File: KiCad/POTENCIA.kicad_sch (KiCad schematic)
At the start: 23 parts, among them J201 Screw_Terminal_01x04, M4 Motor_DC, M5 Motor_DC, M6 Motor_DC, Q201 IRLZ44N, U5 TB6612FNG, U7 ATtiny1616-M, U8 DRV8871DDA

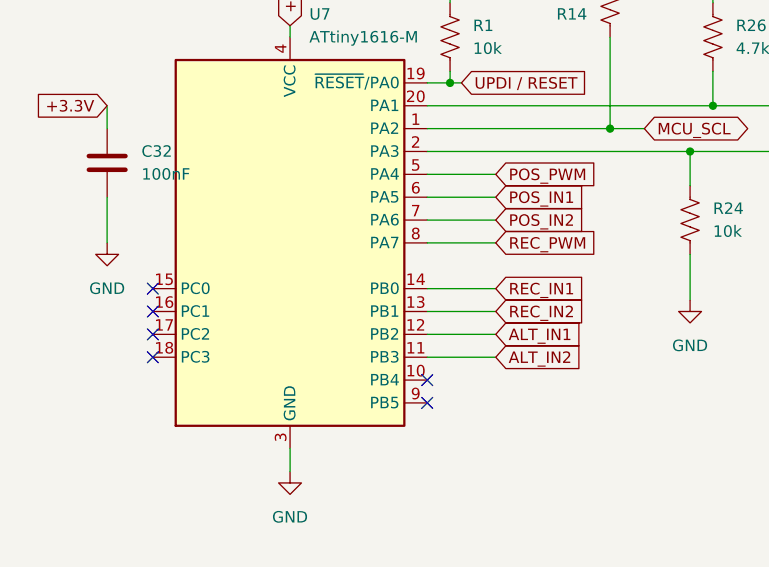
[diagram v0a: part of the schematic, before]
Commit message: Rounting
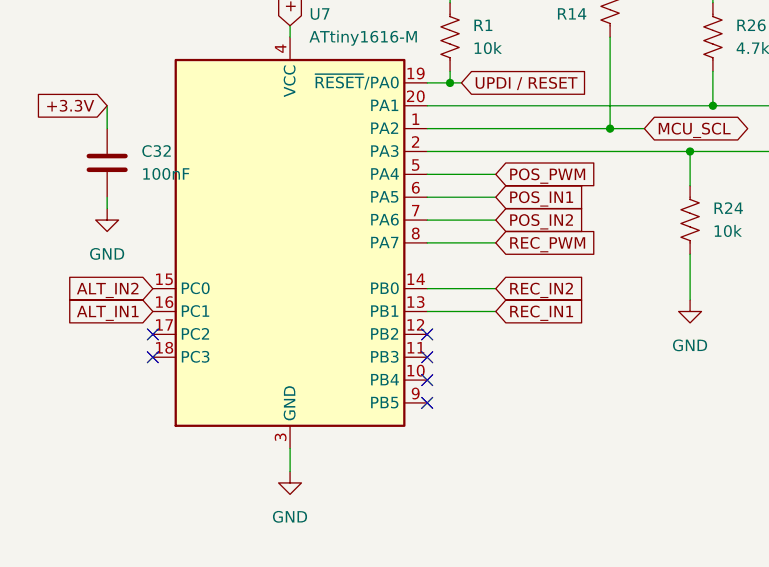
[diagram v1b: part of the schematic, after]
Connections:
- net ALT_IN1: now also U7.16 (PC1); no longer U7.12 (PB2)
- net ALT_IN2: now also U7.15 (PC0); no longer U7.11 (PB3)
- net REC_IN1: now also U7.13 (PB1); no longer U7.14 (PB0)
- net REC_IN2: now also U7.14 (PB0); no longer U7.13 (PB1)
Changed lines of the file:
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@@
 	)
 	(no_connect
-		(at 31.75 152.4)
+		(at 62.23 154.94)
 	)
 	(no_connect
@@
 	)
 	(no_connect
-		(at 31.75 149.86)
-	)
-	(wire
-		(pts
-			(xy 26.67 139.7) (xy 26.67 144.78)
+		(at 62.23 157.48)
+	)
+	(wire
+		(pts
+			(xy 26.67 139.7) (xy 26.67 140.97)
 		)
 		(stroke
@@
 	(wire
 		(pts
-			(xy 62.23 157.48) (xy 69.85 157.48)
-		)
-		(stroke
-			(width 0)
-			(type default)
-		)
-	)
-	(wire
-		(pts
 			(xy 93.98 125.73) (xy 93.98 129.54)
 		)
@@
 		(pts
 			(xy 54.61 88.9) (xy 54.61 95.25)
-		)
-		(stroke
-			(width 0)
-			(type default)
-		)
-	)
-	(wire
-		(pts
-			(xy 62.23 154.94) (xy 69.85 154.94)
 		)
 		(stroke
@@
 	(global_label "REC_IN1"
 		(shape input)
-		(at 69.85 149.86 0)
+		(at 69.85 152.4 0)
 		(fields_autoplaced yes)
 		(effects
@@
 		)
 		(property "Intersheetrefs" "${INTERSHEET_REFS}"
-			(at 80.6366 149.86 0)
+			(at 80.6366 152.4 0)
 			(effects
 				(font
@@
 	(global_label "ALT_IN2"
 		(shape input)
-		(at 69.85 157.48 0)
+		(at 31.75 149.86 180)
+		(fields_autoplaced yes)
+		(effects
+			(font
+				(size 1.27 1.27)
+			)
+			(justify right)
+		)
+		(property "Intersheetrefs" "${INTERSHEET_REFS}"
+			(at 22.2223 149.86 0)
+			(effects
+				(font
+					(size 1.27 1.27)
+				)
+				(justify right)
+				(hide yes)
+			)
+		)
+	)
+	(global_label "VBAT"
+		(shape input)
+		(at 34.29 20.32 180)
+		(fields_autoplaced yes)
+		(effects
+			(font
+				(size 1.27 1.27)
+			)
+			(justify right)
+		)
+		(property "Intersheetrefs" "${INTERSHEET_REFS}"
+			(at 27.5442 20.32 0)
+			(effects
+				(font
+					(size 1.27 1.27)
+				)
+				(justify right)
+				(hide yes)
+			)
+		)
+	)
+	(global_label "POS_IN2"
+		(shape input)
+		(at 69.85 142.24 0)
 		(fields_autoplaced yes)
 		(effects
@@
 		)
 		(property "Intersheetrefs" "${INTERSHEET_REFS}"
-			(at 80.0319 157.48 0)
-			(effects
-				(font
-					(size 1.27 1.27)
-				)
-				(justify left)
-				(hide yes)
-			)
-		)
-	)
-	(global_label "VBAT"
-		(shape input)
-		(at 34.29 20.32 180)
+			(at 80.7576 142.24 0)
+			(effects
+				(font
+					(size 1.27 1.27)
+				)
+				(justify left)
+				(hide yes)
+			)
+		)
+	)
+	(global_label "REC_IN2"
+		(shape input)
+		(at 69.85 149.86 0)
+		(fields_autoplaced yes)
+		(effects
+			(font
+				(size 1.27 1.27)
+			)
+			(justify left)
+		)
+		(property "Intersheetrefs" "${INTERSHEET_REFS}"
+			(at 80.6366 149.86 0)
+			(effects
+				(font
+					(size 1.27 1.27)
+				)
+				(justify left)
+				(hide yes)
+			)
+		)
+	)
+	(global_label "ALT_IN1"
+		(shape input)
+		(at 31.75 152.4 180)
 		(fields_autoplaced yes)
 		(effects
@@
 		)
 		(property "Intersheetrefs" "${INTERSHEET_REFS}"
-			(at 27.5442 20.32 0)
+			(at 22.2223 152.4 0)
 			(effects
 				(font
@@
 				)
 				(justify right)
-				(hide yes)
-			)
-		)
-	)
-	(global_label "POS_IN2"
-		(shape input)
-		(at 69.85 142.24 0)
-		(fields_autoplaced yes)
-		(effects
-			(font
-				(size 1.27 1.27)
-			)
-			(justify left)
-		)
-		(property "Intersheetrefs" "${INTERSHEET_REFS}"
-			(at 80.7576 142.24 0)
-			(effects
-				(font
-					(size 1.27 1.27)
-				)
-				(justify left)
-				(hide yes)
-			)
-		)
-	)
-	(global_label "REC_IN2"
-		(shape input)
-		(at 69.85 152.4 0)
-		(fields_autoplaced yes)
-		(effects
-			(font
-				(size 1.27 1.27)
-			)
-			(justify left)
-		)
-		(property "Intersheetrefs" "${INTERSHEET_REFS}"
-			(at 80.6366 152.4 0)
-			(effects
-				(font
-					(size 1.27 1.27)
-				)
-				(justify left)
-				(hide yes)
-			)
-		)
-	)
-	(global_label "ALT_IN1"
-		(shape input)
-		(at 69.85 154.94 0)
-		(fields_autoplaced yes)
-		(effects
-			(font
-				(size 1.27 1.27)
-			)
-			(justify left)
-		)
-		(property "Intersheetrefs" "${INTERSHEET_REFS}"
-			(at 80.0319 154.94 0)
-			(effects
-				(font
-					(size 1.27 1.27)
-				)
-				(justify left)
 				(hide yes)
 			)
@@
 	(symbol
 		(lib_id "power:GND")
-		(at 26.67 144.78 0)
+		(at 26.67 140.97 0)
 		(unit 1)
 		(exclude_from_sim no)
@@
 		(fields_autoplaced yes)
 		(property "Reference" "#PWR049"
-			(at 26.67 151.13 0)
+			(at 26.67 147.32 0)
 			(effects
 				(font
@@
 		)
 		(property "Value" "GND"
-			(at 26.67 149.86 0)
+			(at 26.67 146.05 0)
 			(effects
 				(font
@@
 		)
 		(property "Footprint" ""
-			(at 26.67 144.78 0)
+			(at 26.67 140.97 0)
 			(effects
 				(font
@@
 		)
 		(property "Datasheet" ""
-			(at 26.67 144.78 0)
+			(at 26.67 140.97 0)
 			(effects
 				(font
@@
 		)
 		(property "Description" "Power symbol creates a global label with name \"GND\" , ground"
-			(at 26.67 144.78 0)
-			(effects
-				(font
+			(at 26.67 140.97 0)
+			(effects
+				(font
